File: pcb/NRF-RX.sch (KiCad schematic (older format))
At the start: 27 parts, among them J1 Conn_01x04_Female, J10 CH7, J11 CH8, J12 CH4, J13 CH4, J2 Conn_01x04_Female, J3 BIND, J4 CH1, J5 CH2, J6 CH3, J7 CH4, J8 CH5, J9 CH6, U1 ATmega328-AU, U2 ATmega328-AU, U3 LM1117-3.3, Y1 Crystal, Y2 Crystal

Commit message: added the updated PCB file for the calculated size
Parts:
- J1, J2: footprint Connector_PinHeader_2.54mm:PinHeader_1x04_P2.54mm_Vertical -> Connector_PinSocket_2.54mm:PinSocket_1x04_P2.54mm_Vertical
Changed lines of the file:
@@
 F 0 "J1" H 3328 6376 50  0000 L CNN
 F 1 "Conn_01x04_Female" H 3328 6285 50  0000 L CNN
-F 2 "Connector_PinHeader_2.54mm:PinHeader_1x04_P2.54mm_Vertical" H 3300 6400 50  0001 C CNN
+F 2 "Connector_PinSocket_2.54mm:PinSocket_1x04_P2.54mm_Vertical" H 3300 6400 50  0001 C CNN
 F 3 "~" H 3300 6400 50  0001 C CNN
 	1    3300 6400
@@
 F 0 "J2" H 3478 6376 50  0000 L CNN
 F 1 "Conn_01x04_Female" H 3478 6285 50  0000 L CNN
-F 2 "Connector_PinHeader_2.54mm:PinHeader_1x04_P2.54mm_Vertical" H 3450 6400 50  0001 C CNN
+F 2 "Connector_PinSocket_2.54mm:PinSocket_1x04_P2.54mm_Vertical" H 3450 6400 50  0001 C CNN
 F 3 "~" H 3450 6400 50  0001 C CNN
 	1    3450 6400

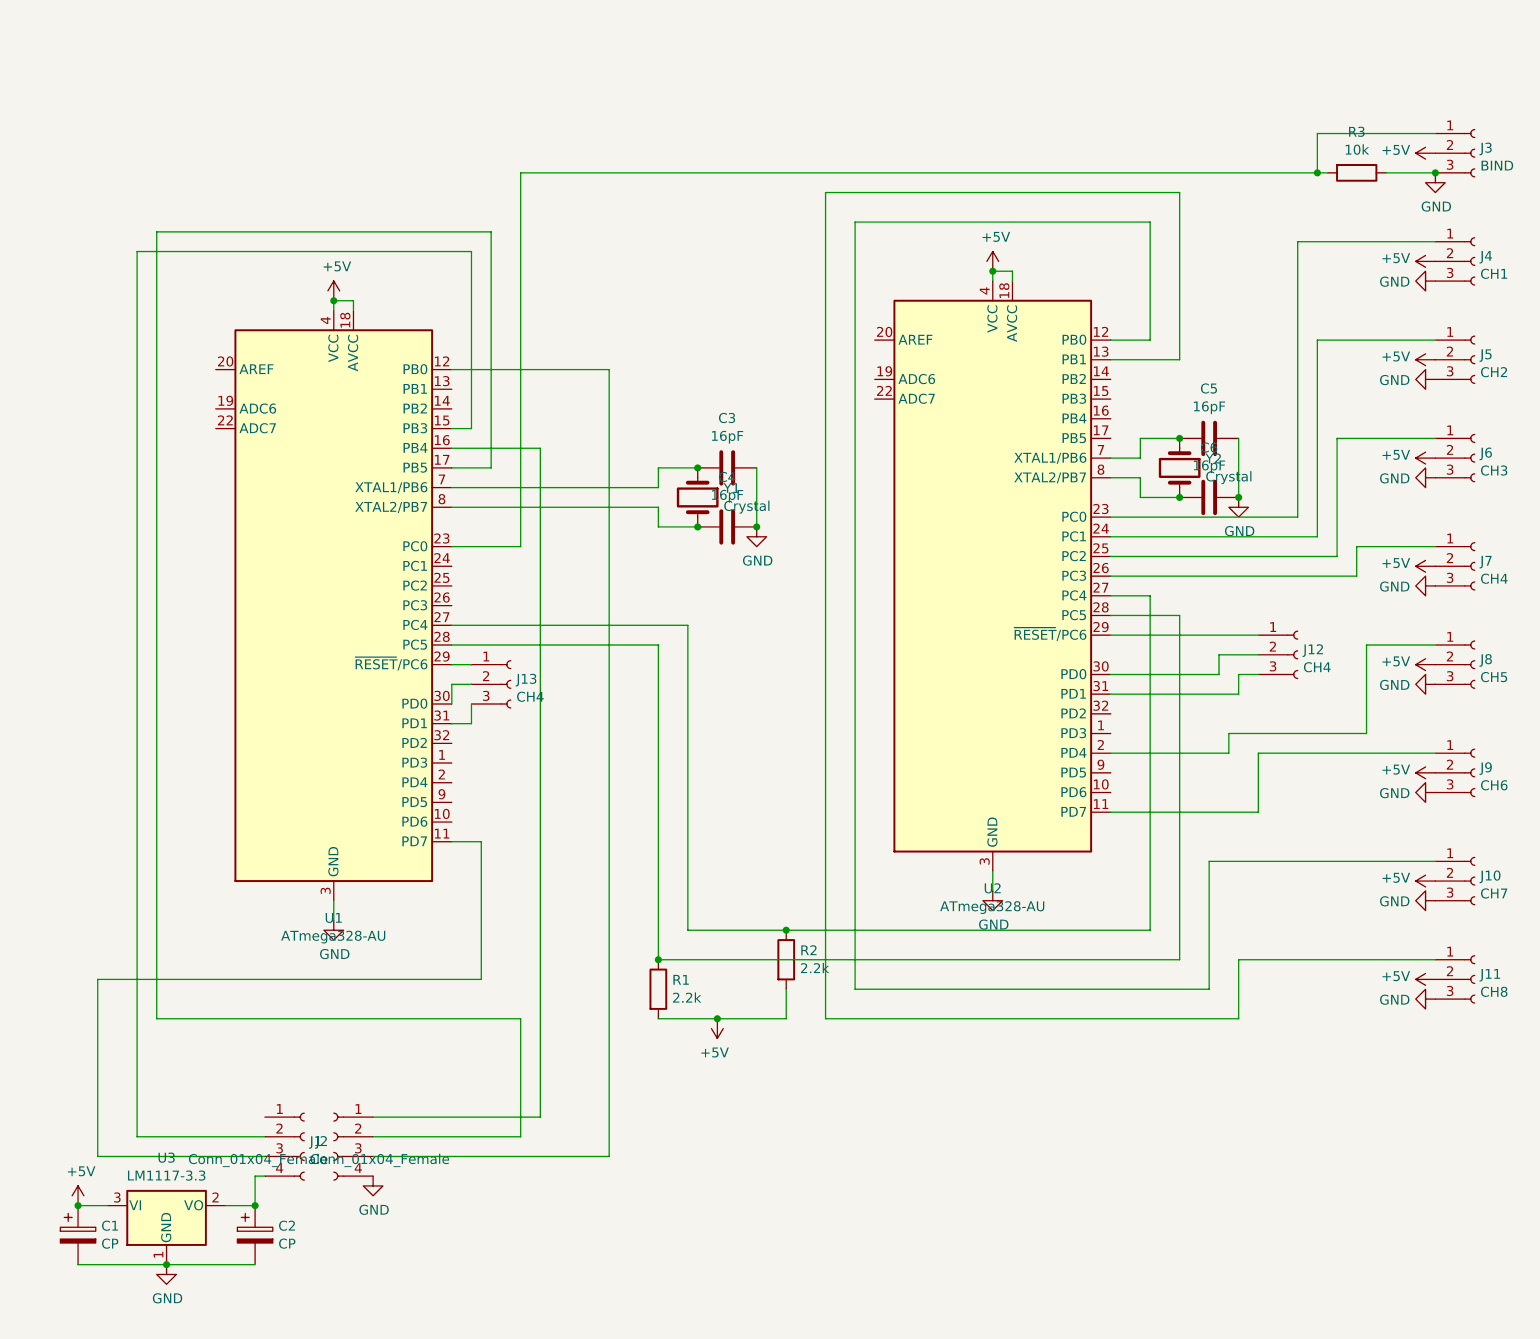
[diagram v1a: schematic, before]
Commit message: added the changes
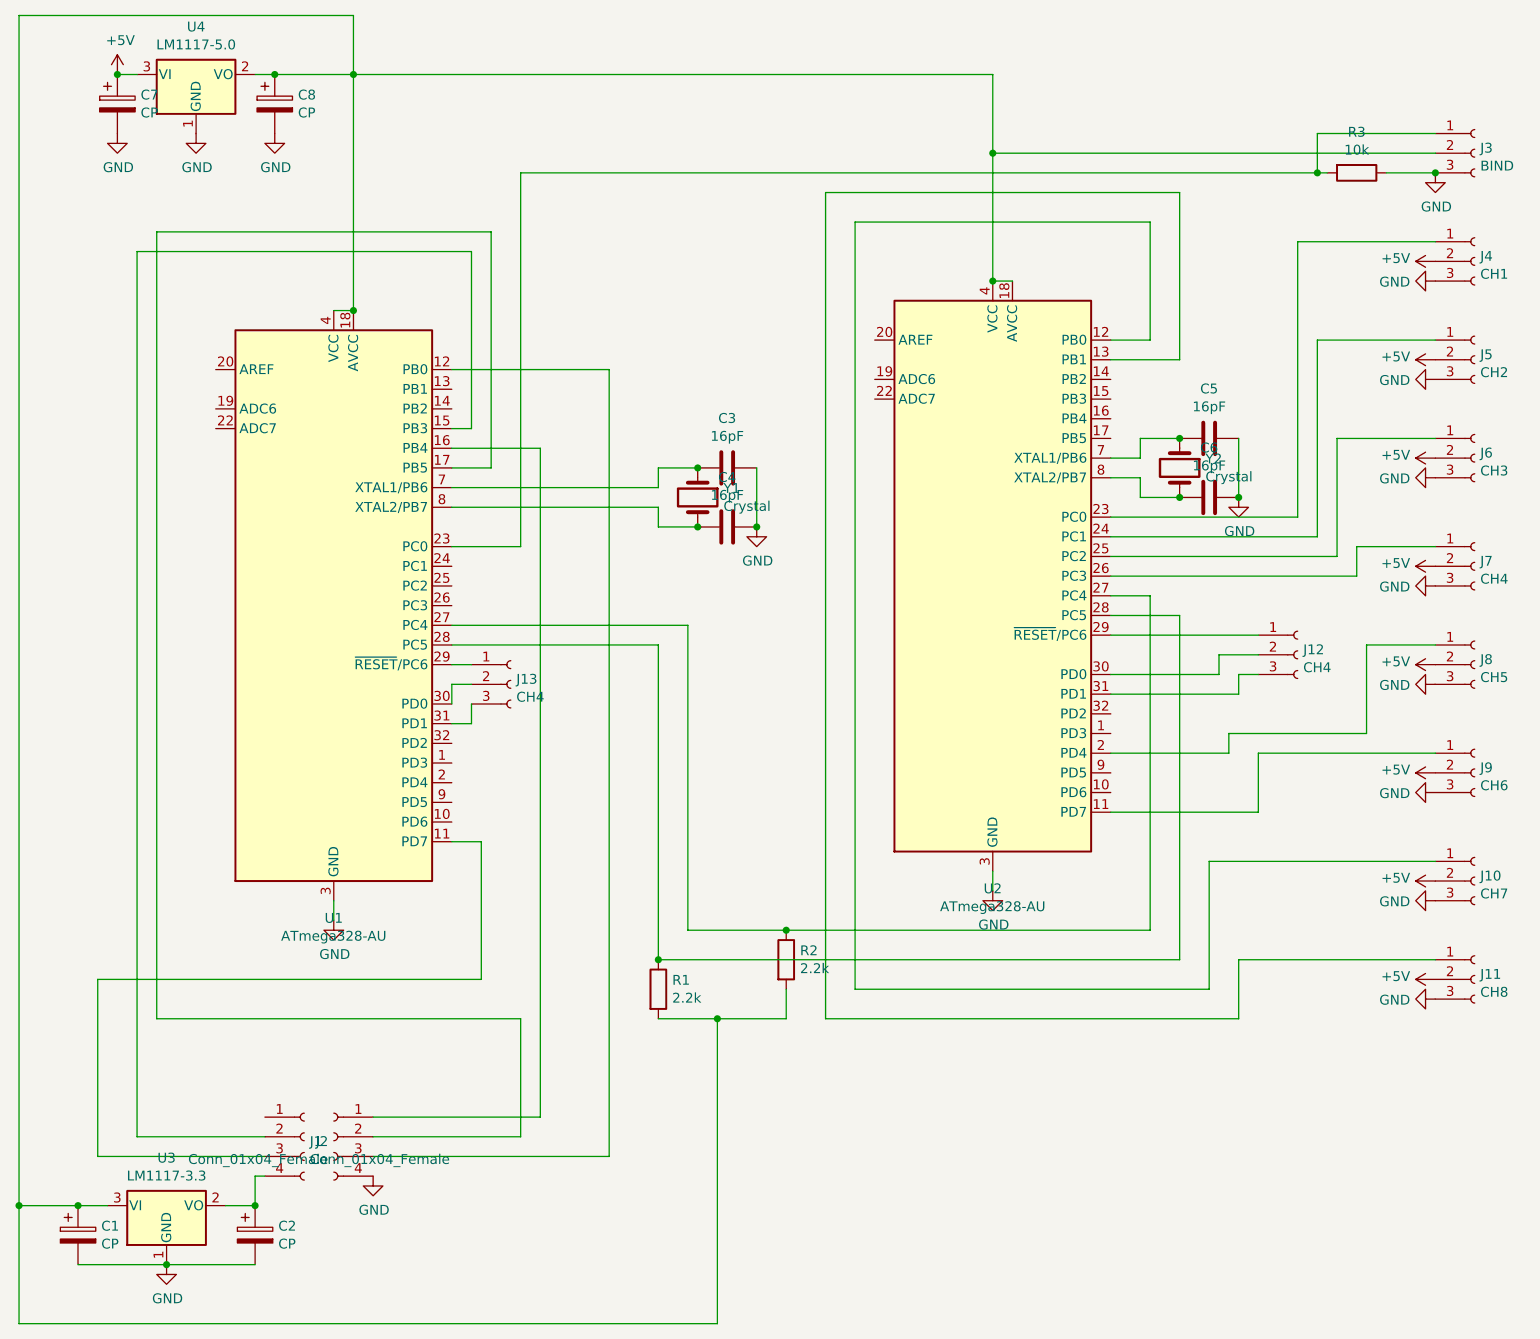
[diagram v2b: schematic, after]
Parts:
- added C7, C8: CP, Capacitor_SMD:CP_Elec_5x5.4, symbol Device:CP
- added U4: LM1117-5.0, Package_TO_SOT_SMD:SOT-223, symbol Regulator_Linear:LM1117-5.0
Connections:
- net +5V: now also C7.1, U4.3 (VI); no longer C1.1, J3.2 (Pin_2), R1.2, R2.2, U1.18 (AVCC), U1.4 (VCC), U1.6 (VCC), U2.18 (AVCC), U2.4 (VCC), U2.6 (VCC), U3.3 (VI)
- net GND: now also C7.2, C8.2, U4.1 (GND)
- new net: C1.1, C8.1, J3.2 (Pin_2), R1.2, R2.2, U1.18 (AVCC), U1.4 (VCC), U1.6 (VCC), U2.18 (AVCC), U2.4 (VCC), U2.6 (VCC), U3.3 (VI), U4.2 (VO)
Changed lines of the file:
@@
 $EndDescr
-$Comp
-L power:+5V #PWR0101
-U 1 1 5F56AD00
-P 3450 2150
-F 0 "#PWR0101" H 3450 2000 50  0001 C CNN
-F 1 "+5V" H 3465 2323 50  0000 C CNN
-F 2 "" H 3450 2150 50  0001 C CNN
-F 3 "" H 3450 2150 50  0001 C CNN
-	1    3450 2150
-	1    0    0    -1
-$EndComp
-Wire Wire Line
-	3450 2200 3450 2150
-Wire Wire Line
-	3450 2150 3550 2150
-Wire Wire Line
-	3550 2150 3550 2200
-Connection ~ 3450 2150
 $Comp
 L power:GND #PWR0102
@@
 	3450 5300 3450 5200
 $Comp
-L MCU_Microchip_ATmega:ATmega328-AU U2
-U 1 1 5F7E3B6B
-P 6800 3550
-F 0 "U2" H 6800 1961 50  0000 C CNN
-F 1 "ATmega328-AU" H 6800 1870 50  0000 C CNN
-F 2 "Package_QFP:TQFP-32_7x7mm_P0.8mm" H 6800 3550 50  0001 C CIN
-F 3 "http://ww1.microchip.com/downloads/en/DeviceDoc/ATmega328_P%20AVR%20MCU%20with%20picoPower%20Technology%20Data%20Sheet%2040001984A.pdf" H 6800 3550 50  0001 C CNN
-	1    6800 3550
-	1    0    0    -1
-$EndComp
-$Comp
-L power:+5V #PWR0103
-U 1 1 5F7E3B71
-P 6800 2000
-F 0 "#PWR0103" H 6800 1850 50  0001 C CNN
-F 1 "+5V" H 6815 2173 50  0000 C CNN
-F 2 "" H 6800 2000 50  0001 C CNN
-F 3 "" H 6800 2000 50  0001 C CNN
-	1    6800 2000
-	1    0    0    -1
-$EndComp
-Wire Wire Line
-	6800 2050 6800 2000
-Wire Wire Line
-	6800 2000 6900 2000
-Wire Wire Line
-	6900 2000 6900 2050
-Connection ~ 6800 2000
-$Comp
 L power:GND #PWR0104
 U 1 1 5F7E3B7B
@@
 Connection ~ 8050 3150
 Wire Wire Line
-	7400 2950 7550 2950
-Wire Wire Line
 	7550 2950 7550 2850
 Wire Wire Line
@@
 	5750 5350 7600 5350
 Wire Wire Line
-	5100 5800 5400 5800
-Wire Wire Line
 	5750 5800 5750 5650
-$Comp
-L power:+5V #PWR0109
-U 1 1 5F822335
-P 5400 5800
-F 0 "#PWR0109" H 5400 5650 50  0001 C CNN
-F 1 "+5V" H 5415 5973 50  0000 C CNN
-F 2 "" H 5400 5800 50  0001 C CNN
-F 3 "" H 5400 5800 50  0001 C CNN
-	1    5400 5800
-	-1   0    0    1
-$EndComp
-Connection ~ 5400 5800
-Wire Wire Line
-	5400 5800 5750 5800
 Wire Wire Line
 	7600 5350 7600 3650
-Wire Wire Line
-	7600 3650 7400 3650
-Wire Wire Line
-	7400 3750 7750 3750
 Wire Wire Line
 	7750 3750 7750 5500
@@
 	1    0    0    -1
 $EndComp
-$Comp
-L power:+5V #PWR0106
-U 1 1 5F8735EA
-P 2150 6750
-F 0 "#PWR0106" H 2150 6600 50  0001 C CNN
-F 1 "+5V" H 2165 6923 50  0000 C CNN
-F 2 "" H 2150 6750 50  0001 C CNN
-F 3 "" H 2150 6750 50  0001 C CNN
-	1    2150 6750
-	1    0    0    -1
-$EndComp
-Connection ~ 2150 6750
 $Comp
 L power:GND #PWR0110
@@
 $EndComp
 $Comp
-L power:+5V #PWR0120
-U 1 1 5F889936
-P 9050 1400
-F 0 "#PWR0120" H 9050 1250 50  0001 C CNN
-F 1 "+5V" V 9065 1528 50  0000 L CNN
-F 2 "" H 9050 1400 50  0001 C CNN
-F 3 "" H 9050 1400 50  0001 C CNN
-	1    9050 1400
-	0    -1   -1   0
-$EndComp
-$Comp
 L power:+5V #PWR0121
 U 1 1 5F88B088
@@
 	8450 1500 8500 1500
 Wire Wire Line
-	7400 3250 8350 3250
-Wire Wire Line
 	8350 1850 9050 1850
 Wire Wire Line
-	7400 3350 8450 3350
-Wire Wire Line
 	8450 3350 8450 2350
 Wire Wire Line
 	8450 2350 9050 2350
 Wire Wire Line
-	7400 3450 8550 3450
-Wire Wire Line
 	8550 3450 8550 2850
 Wire Wire Line
 	8550 2850 9050 2850
 Wire Wire Line
-	7400 3550 8650 3550
-Wire Wire Line
 	8650 3550 8650 3400
 Wire Wire Line
 	8650 3400 9050 3400
 Wire Wire Line
-	7400 4450 8000 4450
-Wire Wire Line
 	7400 4750 8150 4750
 Wire Wire Line
@@
 	8350 3250 8350 1850
 Wire Wire Line
-	7400 2350 7600 2350
-Wire Wire Line
 	7600 2350 7600 1750
 Wire Wire Line
-	7600 1750 6100 1750
-Wire Wire Line
 	6100 1750 6100 5650
 Wire Wire Line
@@
 Wire Wire Line
 	7900 5000 9050 5000
-Wire Wire Line
-	7400 2450 7750 2450
 Wire Wire Line
 	7750 2450 7750 1600
@@
 	7400 3850 8150 3850
 Wire Wire Line
-	7400 4050 7950 4050
-Wire Wire Line
 	7950 4050 7950 3950
 Wire Wire Line
 	7950 3950 8150 3950
-Wire Wire Line
-	7400 4150 8050 4150
 Wire Wire Line
 	8050 4150 8050 4050
@@
 Wire Wire Line
 	4150 4300 4150 4200
+$Comp
+L Regulator_Linear:LM1117-5.0 U4
+U 1 1 5F976E32
+P 2750 1000
+F 0 "U4" H 2750 1242 50  0000 C CNN
+F 1 "LM1117-5.0" H 2750 1151 50  0000 C CNN
+F 2 "Package_TO_SOT_SMD:SOT-223" H 2750 1000 50  0001 C CNN
+F 3 "http://www.ti.com/lit/ds/symlink/lm1117.pdf" H 2750 1000 50  0001 C CNN
+	1    2750 1000
+	1    0    0    -1
+$EndComp
+$Comp
+L Device:CP C7
+U 1 1 5F97C8CA
+P 2350 1150
+F 0 "C7" H 2468 1196 50  0000 L CNN
+F 1 "CP" H 2468 1105 50  0000 L CNN
+F 2 "Capacitor_SMD:CP_Elec_5x5.4" H 2388 1000 50  0001 C CNN
+F 3 "~" H 2350 1150 50  0001 C CNN
+	1    2350 1150
+	1    0    0    -1
+$EndComp
+$Comp
+L Device:CP C8
+U 1 1 5F97DA5B
+P 3150 1150
+F 0 "C8" H 3268 1196 50  0000 L CNN
+F 1 "CP" H 3268 1105 50  0000 L CNN
+F 2 "Capacitor_SMD:CP_Elec_5x5.4" H 3188 1000 50  0001 C CNN
+F 3 "~" H 3150 1150 50  0001 C CNN
+	1    3150 1150
+	1    0    0    -1
+$EndComp
+Wire Wire Line
+	2350 1000 2450 1000
+Wire Wire Line
+	3050 1000 3150 1000
+$Comp
+L power:GND #PWR0101
+U 1 1 5F9944E4
+P 2350 1300
+F 0 "#PWR0101" H 2350 1050 50  0001 C CNN
+F 1 "GND" H 2355 1127 50  0000 C CNN
+F 2 "" H 2350 1300 50  0001 C CNN
+F 3 "" H 2350 1300 50  0001 C CNN
+	1    2350 1300
+	1    0    0    -1
+$EndComp
+$Comp
+L power:GND #PWR0103
+U 1 1 5F994CDC
+P 2750 1300
+F 0 "#PWR0103" H 2750 1050 50  0001 C CNN
+F 1 "GND" H 2755 1127 50  0000 C CNN
+F 2 "" H 2750 1300 50  0001 C CNN
+F 3 "" H 2750 1300 50  0001 C CNN
+	1    2750 1300
+	1    0    0    -1
+$EndComp
+$Comp
+L power:GND #PWR0129
+U 1 1 5F99548C
+P 3150 1300
+F 0 "#PWR0129" H 3150 1050 50  0001 C CNN
+F 1 "GND" H 3155 1127 50  0000 C CNN
+F 2 "" H 3150 1300 50  0001 C CNN
+F 3 "" H 3150 1300 50  0001 C CNN
+	1    3150 1300
+	1    0    0    -1
+$EndComp
+$Comp
+L power:+5V #PWR0130
+U 1 1 5F995B13
+P 2350 1000
+F 0 "#PWR0130" H 2350 850 50  0001 C CNN
+F 1 "+5V" H 2365 1173 50  0000 C CNN
+F 2 "" H 2350 1000 50  0001 C CNN
+F 3 "" H 2350 1000 50  0001 C CNN
+	1    2350 1000
+	1    0    0    -1
+$EndComp
+Connection ~ 2350 1000
+Wire Wire Line
+	7600 1750 6100 1750
+Wire Wire Line
+	7400 4450 8000 4450
+Wire Wire Line
+	7400 4150 8050 4150
+Wire Wire Line
+	7400 4050 7950 4050
+Wire Wire Line
+	7400 3750 7750 3750
+Wire Wire Line
+	7600 3650 7400 3650
+Wire Wire Line
+	7400 3550 8650 3550
+Wire Wire Line
+	7400 3450 8550 3450
+Wire Wire Line
+	7400 3350 8450 3350
+Wire Wire Line
+	7400 3250 8350 3250
+Wire Wire Line
+	7400 2950 7550 2950
+Wire Wire Line
+	7400 2450 7750 2450
+Wire Wire Line
+	7400 2350 7600 2350
+$Comp
+L MCU_Microchip_ATmega:ATmega328-AU U2
+U 1 1 5F7E3B6B
+P 6800 3550
+F 0 "U2" H 6800 1961 50  0000 C CNN
+F 1 "ATmega328-AU" H 6800 1870 50  0000 C CNN
+F 2 "Package_QFP:TQFP-32_7x7mm_P0.8mm" H 6800 3550 50  0001 C CIN
+F 3 "http://ww1.microchip.com/downloads/en/DeviceDoc/ATmega328_P%20AVR%20MCU%20with%20picoPower%20Technology%20Data%20Sheet%2040001984A.pdf" H 6800 3550 50  0001 C CNN
+	1    6800 3550
+	1    0    0    -1
+$EndComp
+Wire Wire Line
+	6900 2050 6800 2050
+Wire Wire Line
+	6800 2050 6800 1400
+Wire Wire Line
+	6800 1000 3550 1000
+Connection ~ 6800 2050
+Connection ~ 3150 1000
+Wire Wire Line
+	3450 2200 3550 2200
+Wire Wire Line
+	3550 2200 3550 1000
+Connection ~ 3550 2200
+Connection ~ 3550 1000
+Wire Wire Line
+	3550 1000 3150 1000
+Wire Wire Line
+	3550 1000 3550 700
+Wire Wire Line
+	3550 700  1850 700
+Wire Wire Line
+	1850 700  1850 6750
+Wire Wire Line
+	1850 6750 2150 6750
+Connection ~ 2150 6750
+Wire Wire Line
+	5100 5800 5400 5800
+Wire Wire Line
+	5400 5800 5400 7350
+Wire Wire Line
+	5400 7350 1850 7350
+Wire Wire Line
+	1850 7350 1850 6750
+Connection ~ 5400 5800
+Wire Wire Line
+	5400 5800 5750 5800
+Connection ~ 1850 6750
+Wire Wire Line
+	9050 1400 6800 1400
+Connection ~ 6800 1400
+Wire Wire Line
+	6800 1400 6800 1000
 $EndSCHEMATC
